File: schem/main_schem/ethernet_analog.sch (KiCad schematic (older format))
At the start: 11 parts, among them U1 SPDT_ANALOG, U2 SPDT_ANALOG

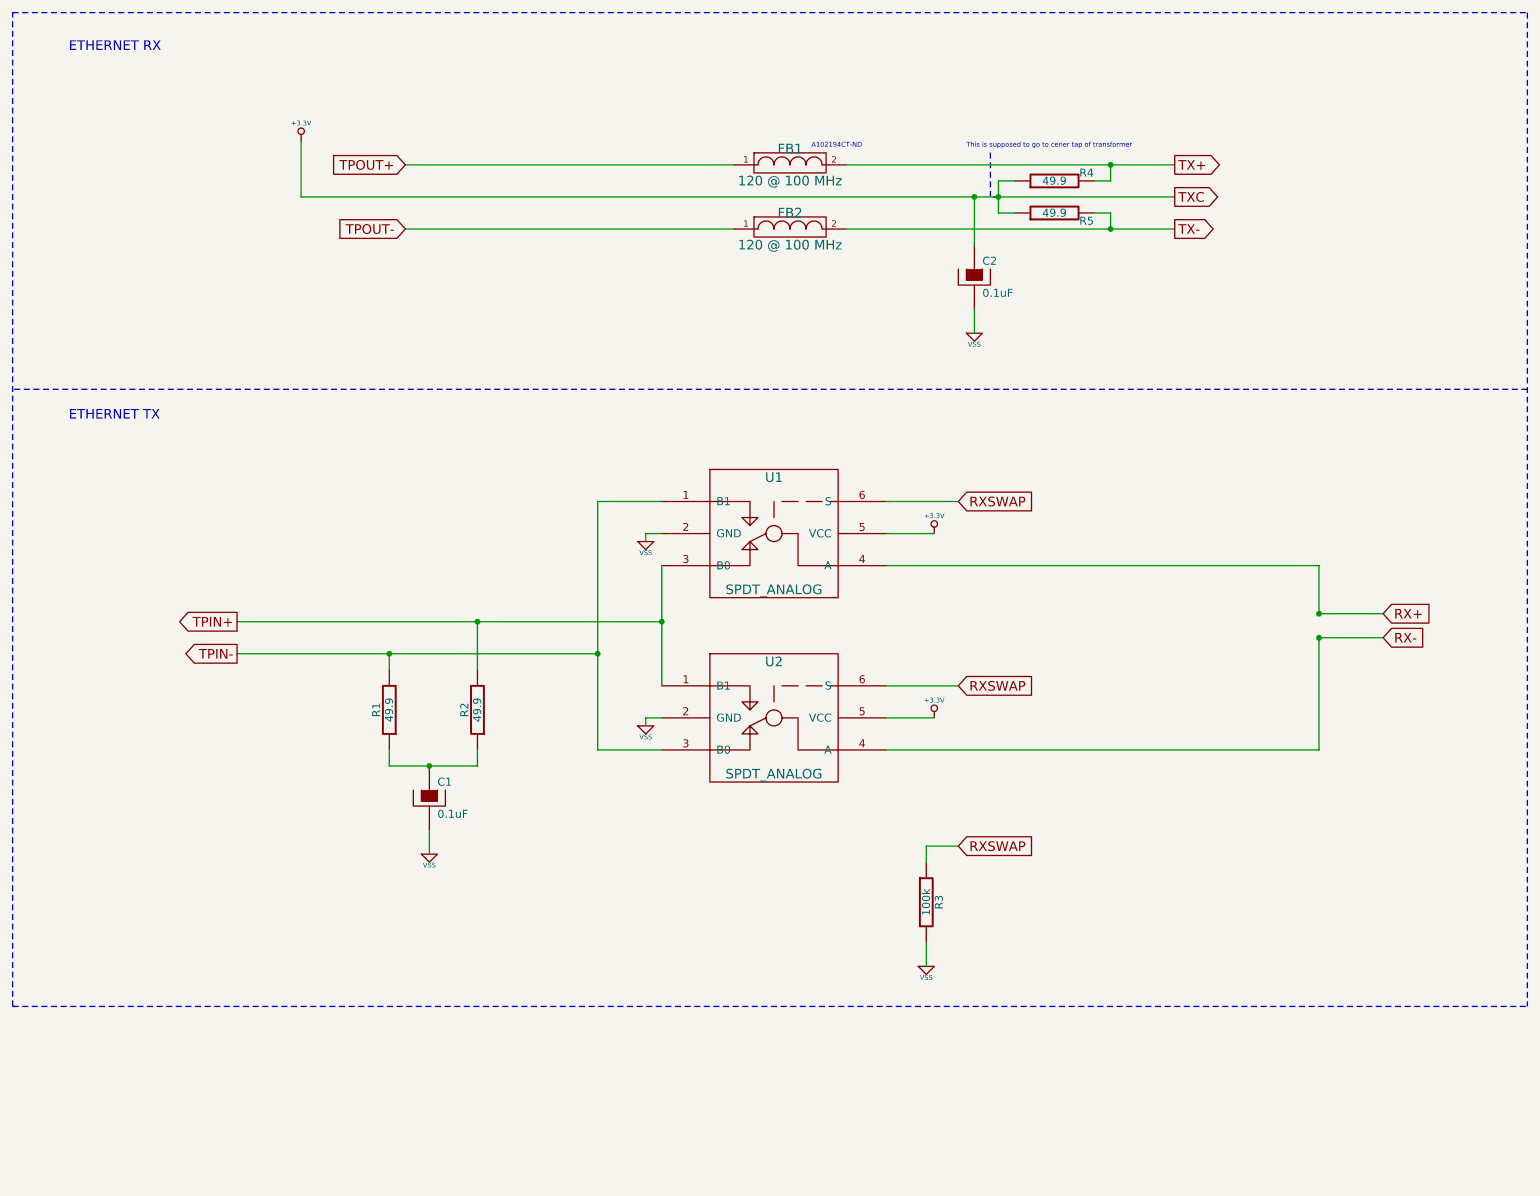
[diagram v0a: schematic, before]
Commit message: save schematics
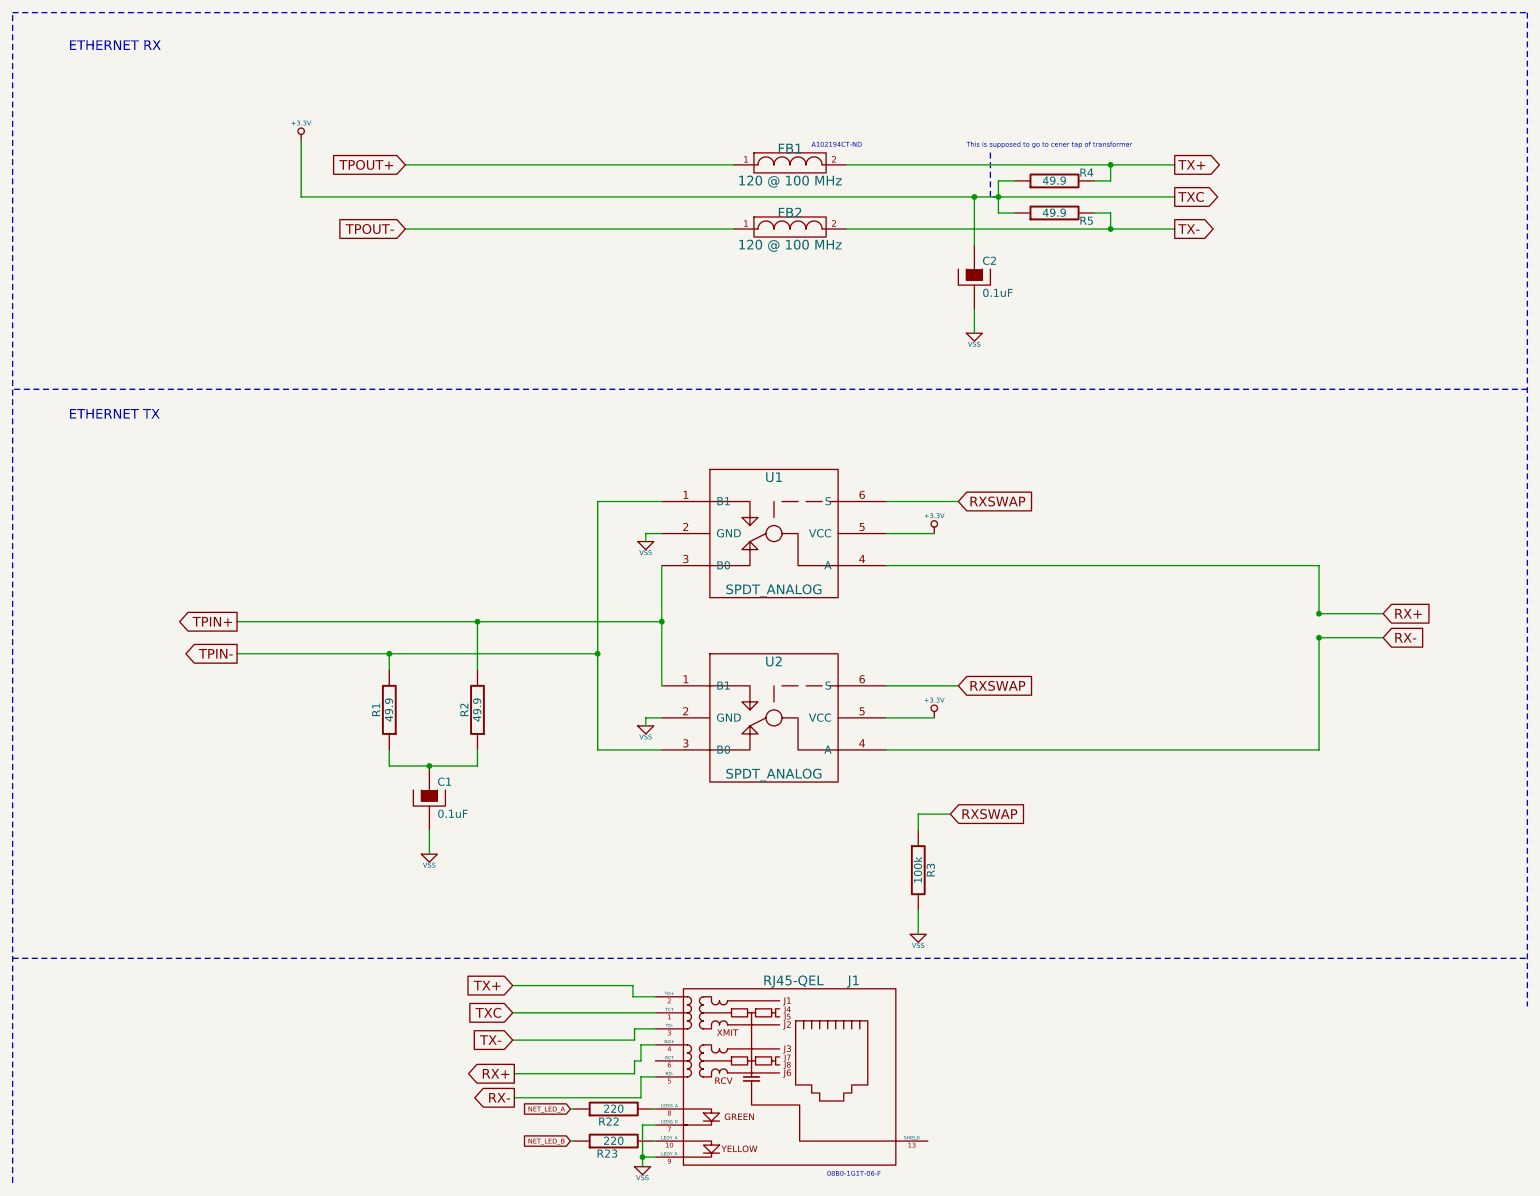
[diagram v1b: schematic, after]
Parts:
- added J1: RJ45-QEL, symbol RJ45-QEL
- added R22, R23: 220, symbol R
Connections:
- net +3.3V: now also J1.1 (TCT)
- net RX+: now also J1.4 (RD+)
- net RX-: now also J1.5 (RD-)
- net TX+: now also J1.2 (TD+)
- net TX-: now also J1.3 (TD-)
- net VSS: now also J1.7 (LEDG_K), J1.9 (LEDY_K)
- new net: J1.10 (LEDY_A), R23.2
- new net: J1.8 (LEDG_A), R22.2
- new net NET_LED_A: R22.1
- new net NET_LED_B: R23.1
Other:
- note added: "08B0-1G1T-06-F"
- moved on the sheet: R3
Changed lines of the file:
@@
-EESchema Schematic File Version 2  date 10/17/2012 8:53:55 AM
+EESchema Schematic File Version 2  date 10/20/2012 6:17:28 PM
 LIBS:power
 LIBS:device
@@
 Sheet 2 6
 Title "Ethernet Analog Subsystem w/ Polarity Switching"
-Date "17 oct 2012"
+Date "20 oct 2012"
 Rev ""
 Comp "Ingersoll Rand 402 Group"
@@
 Comment4 ""
 $EndDescr
-Wire Notes Line
-	1150 6700 10600 6700
+Wire Wire Line
+	4630 7540 4650 7540
+Wire Wire Line
+	4650 7340 4630 7340
+Connection ~ 5080 7640
+Wire Wire Line
+	5160 7640 5080 7640
+Wire Wire Line
+	5070 7040 5030 7040
+Wire Wire Line
+	5070 7040 5070 6940
+Wire Wire Line
+	5070 6940 5160 6940
+Wire Wire Line
+	5030 7040 5030 7120
+Wire Wire Line
+	5030 7120 4280 7120
+Wire Wire Line
+	4270 6740 5160 6740
+Wire Notes Line
+	1150 7800 1150 500
 Wire Notes Line
 	10600 2850 1150 2850
@@
 	9300 5100 6600 5100
 Wire Wire Line
-	7050 5700 6850 5700
-Wire Wire Line
-	6850 5700 6850 5800
+	7000 5500 6800 5500
+Wire Wire Line
+	6800 5500 6800 5600
 Wire Wire Line
 	6600 4700 7050 4700
@@
 	6600 3550 7050 3550
 Wire Wire Line
-	6850 6300 6850 6450
+	6800 6100 6800 6250
 Wire Wire Line
 	6600 3950 9300 3950
@@
 Connection ~ 9300 4250
 Wire Wire Line
-	5200 4300 2550 4300
-Wire Wire Line
-	4800 4500 2550 4500
+	2550 4300 5200 4300
+Wire Wire Line
+	2550 4500 4800 4500
 Wire Wire Line
 	4800 5100 5200 5100
@@
 Connection ~ 8000 1850
 Wire Notes Line
-	1150 6700 1150 500
-Wire Notes Line
 	1150 500  10600 500
 Wire Notes Line
 	10600 500  10600 6700
+Wire Notes Line
+	1150 6400 10600 6400
+Wire Wire Line
+	4270 6570 5020 6570
+Wire Wire Line
+	5020 6570 5020 6640
+Wire Wire Line
+	5020 6640 5160 6640
+Wire Wire Line
+	5030 6910 5030 6840
+Wire Wire Line
+	5030 6910 4270 6910
+Wire Wire Line
+	4280 7270 5070 7270
+Wire Wire Line
+	5070 7270 5070 7140
+Wire Wire Line
+	5070 7140 5160 7140
+Wire Wire Line
+	5030 6840 5160 6840
+Wire Wire Line
+	5160 7440 5080 7440
+Wire Wire Line
+	5080 7440 5080 7700
+Wire Wire Line
+	5150 7340 5160 7340
+Wire Wire Line
+	5160 7540 5150 7540
+Text GLabel 4630 7540 0    30   Input ~ 0
+NET_LED_B
+$Comp
+L R R23
+U 1 1 5082E53A
+P 4900 7540
+F 0 "R23" V 4820 7580 50  0000 C CNN
+F 1 "220" V 4900 7540 50  0000 C CNN
+	1    4900 7540
+	0    -1   -1   0
+$EndComp
+$Comp
+L R R22
+U 1 1 5082E45D
+P 4900 7340
+F 0 "R22" V 4820 7370 50  0000 C CNN
+F 1 "220" V 4900 7340 50  0000 C CNN
+	1    4900 7340
+	0    -1   -1   0
+$EndComp
+Text GLabel 4630 7340 0    30   Input ~ 0
+NET_LED_A
+Text Notes 6230 7770 0    30   ~ 0
+08B0-1G1T-06-F
+$Comp
+L VSS #PWR3
+U 1 1 5082E2BE
+P 5080 7700
+F 0 "#PWR3" H 5080 7700 30  0001 C CNN
+F 1 "VSS" H 5080 7630 30  0000 C CNN
+	1    5080 7700
+	1    0    0    -1
+$EndComp
+Text GLabel 4280 7120 0    60   Output ~ 0
+RX+
+Text GLabel 4280 7270 0    60   Output ~ 0
+RX-
+Text GLabel 4270 6570 0    60   Input ~ 0
+TX+
+Text GLabel 4270 6910 0    60   Input ~ 0
+TX-
+Text GLabel 4270 6740 0    60   Input ~ 0
+TXC
+$Comp
+L RJ45-QEL J1
+U 1 1 5082E1D8
+P 6260 7140
+F 0 "J1" H 6360 7740 60  0000 L CNN
+F 1 "RJ45-QEL" H 6210 7740 60  0000 R CNN
+	1    6260 7140
+	1    0    0    -1
+$EndComp
 Text Notes 1500 750  0    60   ~ 0
 ETHERNET RX
@@
 ETHERNET TX
 $Comp
-L +3.3V #PWR01
+L +3.3V #PWR1
 U 1 1 507229A7
 P 2950 1300
-F 0 "#PWR01" H 2950 1260 30  0001 C CNN
+F 0 "#PWR1" H 2950 1260 30  0001 C CNN
 F 1 "+3.3V" H 2950 1410 30  0000 C CNN
 	1    2950 1300
@@
 This is supposed to go to cener tap of transformer
 $Comp
-L VSS #PWR02
+L VSS #PWR9
 U 1 1 506EFD34
 P 7150 2500
-F 0 "#PWR02" H 7150 2500 30  0001 C CNN
+F 0 "#PWR9" H 7150 2500 30  0001 C CNN
 F 1 "VSS" H 7150 2430 30  0000 C CNN
 	1    7150 2500
@@
 $EndComp
 $Comp
-L VSS #PWR03
+L VSS #PWR2
 U 1 1 506EFD0E
 P 3750 5750
-F 0 "#PWR03" H 3750 5750 30  0001 C CNN
+F 0 "#PWR2" H 3750 5750 30  0001 C CNN
 F 1 "VSS" H 3750 5680 30  0000 C CNN
 	1    3750 5750
@@
 $EndComp
 $Comp
-L VSS #PWR04
+L VSS #PWR6
 U 1 1 506EFADF
-P 6850 6450
-F 0 "#PWR04" H 6850 6450 30  0001 C CNN
-F 1 "VSS" H 6850 6380 30  0000 C CNN
-	1    6850 6450
+P 6800 6250
+F 0 "#PWR6" H 6800 6250 30  0001 C CNN
+F 1 "VSS" H 6800 6180 30  0000 C CNN
+	1    6800 6250
 	1    0    0    -1
 $EndComp
@@
 L R R3
 U 1 1 506EFAD8
-P 6850 6050
-F 0 "R3" V 6930 6050 50  0000 C CNN
-F 1 "100k" V 6850 6050 50  0000 C CNN
-	1    6850 6050
-	1    0    0    -1
-$EndComp
-Text GLabel 7050 5700 2    60   Input ~ 0
+P 6800 5850
+F 0 "R3" V 6880 5850 50  0000 C CNN
+F 1 "100k" V 6800 5850 50  0000 C CNN
+	1    6800 5850
+	1    0    0    -1
+$EndComp
+Text GLabel 7000 5500 2    60   Input ~ 0
 RXSWAP
 Text GLabel 7050 4700 2    60   Input ~ 0
@@
 RXSWAP
 $Comp
-L VSS #PWR05
+L VSS #PWR4
 U 1 1 506EFA1F
 P 5100 3800
-F 0 "#PWR05" H 5100 3800 30  0001 C CNN
+F 0 "#PWR4" H 5100 3800 30  0001 C CNN
 F 1 "VSS" H 5100 3730 30  0000 C CNN
 	1    5100 3800
@@
 $EndComp
 $Comp
-L VSS #PWR06
+L VSS #PWR5
 U 1 1 506EF9D4
 P 5100 4950
-F 0 "#PWR06" H 5100 4950 30  0001 C CNN
+F 0 "#PWR5" H 5100 4950 30  0001 C CNN
 F 1 "VSS" H 5100 4880 30  0000 C CNN
 	1    5100 4950
@@
 $EndComp
 $Comp
-L +3.3V #PWR07
+L +3.3V #PWR8
 U 1 1 506EF9AE
 P 6900 4900
-F 0 "#PWR07" H 6900 4860 30  0001 C CNN
+F 0 "#PWR8" H 6900 4860 30  0001 C CNN
 F 1 "+3.3V" H 6900 5010 30  0000 C CNN
 	1    6900 4900
@@
 $EndComp
 $Comp
-L +3.3V #PWR08
+L +3.3V #PWR7
 U 1 1 506EF99F
 P 6900 3750
-F 0 "#PWR08" H 6900 3710 30  0001 C CNN
+F 0 "#PWR7" H 6900 3710 30  0001 C CNN
 F 1 "+3.3V" H 6900 3860 30  0000 C CNN
 	1    6900 3750
